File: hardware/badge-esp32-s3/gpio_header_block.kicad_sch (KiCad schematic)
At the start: 2 parts, among them J7 SD Card, U20 2x14_female

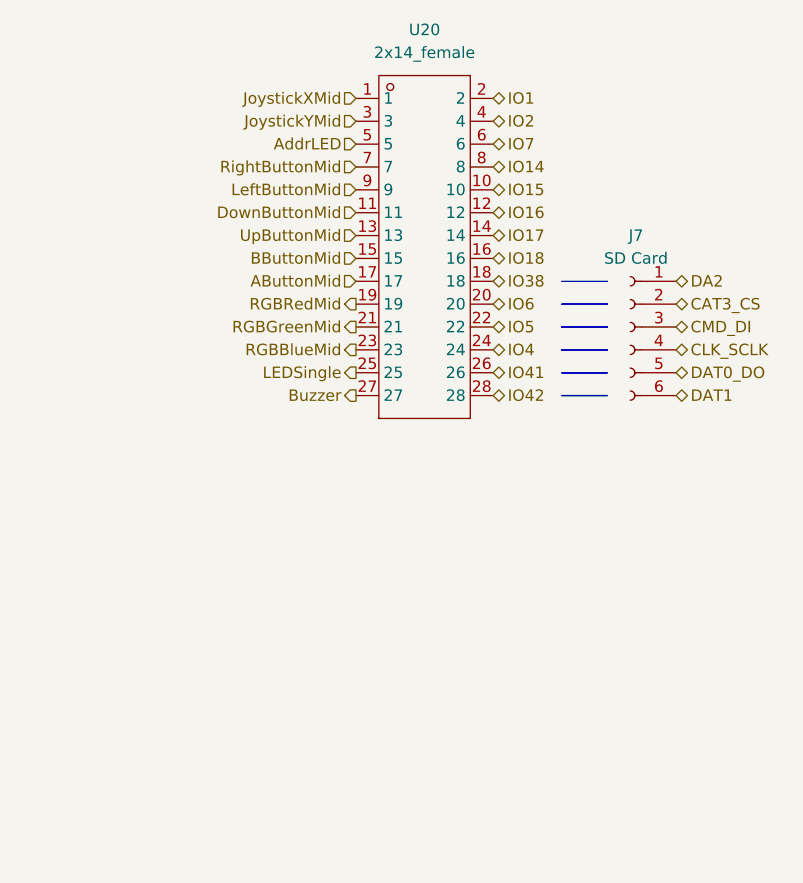
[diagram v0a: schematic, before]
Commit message: almost finished
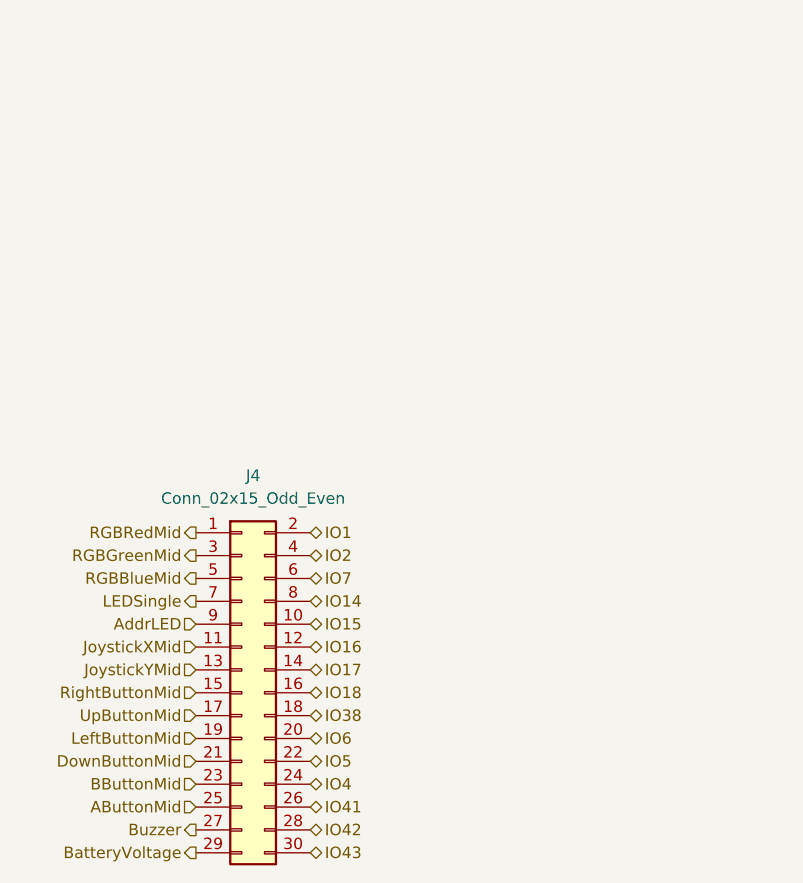
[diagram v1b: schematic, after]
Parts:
- removed J7: SD Card, symbol Connector:Conn_01x06_Socket
- removed U20: 2x14_female, lcsc-lib:HDR-TH_28P-P2.54-V-F-R2-C14-S2.54, symbol lcsc-lib:HX PM2.54-2X14P ZC
- added J4: Conn_02x15_Odd_Even, Connector_PinHeader_2.54mm:PinHeader_2x15_P2.54mm_Vertical, symbol Connector_Generic:Conn_02x15_Odd_Even
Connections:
- net AButtonMid: now also J4.25 (Pin_25)
- net AddrLED: now also J4.9 (Pin_9)
- net BButtonMid: now also J4.23 (Pin_23)
- net Buzzer: now also J4.27 (Pin_27)
- net DownButtonMid: now also J4.21 (Pin_21)
- net IO1: now also J4.2 (Pin_2)
- net IO14: now also J4.8 (Pin_8)
- net IO15: now also J4.10 (Pin_10)
- net IO16: now also J4.12 (Pin_12)
- net IO17: now also J4.14 (Pin_14)
- net IO18: now also J4.16 (Pin_16)
- net IO2: now also J4.4 (Pin_4)
- net IO38: now also J4.18 (Pin_18)
- net IO4: now also J4.24 (Pin_24)
- net IO41: now also J4.26 (Pin_26)
- net IO42: now also J4.28 (Pin_28)
- net IO5: now also J4.22 (Pin_22)
- net IO6: now also J4.20 (Pin_20)
- net IO7: now also J4.6 (Pin_6)
- net JoystickXMid: now also J4.11 (Pin_11)
- net JoystickYMid: now also J4.13 (Pin_13)
- net LEDSingle: now also J4.7 (Pin_7)
- net LeftButtonMid: now also J4.19 (Pin_19)
- net RGBBlueMid: now also J4.5 (Pin_5)
- net RGBGreenMid: now also J4.3 (Pin_3)
- net RGBRedMid: now also J4.1 (Pin_1)
- net RightButtonMid: now also J4.15 (Pin_15)
- net UpButtonMid: now also J4.17 (Pin_17)
- new net BatteryVoltage: J4.29 (Pin_29)
- new net IO43: J4.30 (Pin_30)
